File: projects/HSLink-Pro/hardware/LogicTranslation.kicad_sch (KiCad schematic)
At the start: 41 parts, among them U11 SN74LVC1T45DCK, U12 SN74LVC1T45DCK, U2 SN74LVC1T45DCK, U3 SN74LVC1T45DCK, U4 SN74LVC1T45DCK, U5 SN74LVC1T45DCK, U6 SN74LVC1T45DCK, U7 SN74LVC1T45DCK, U8 SN74LVC1T45DCK, U9 SN74LVC1T45DCK

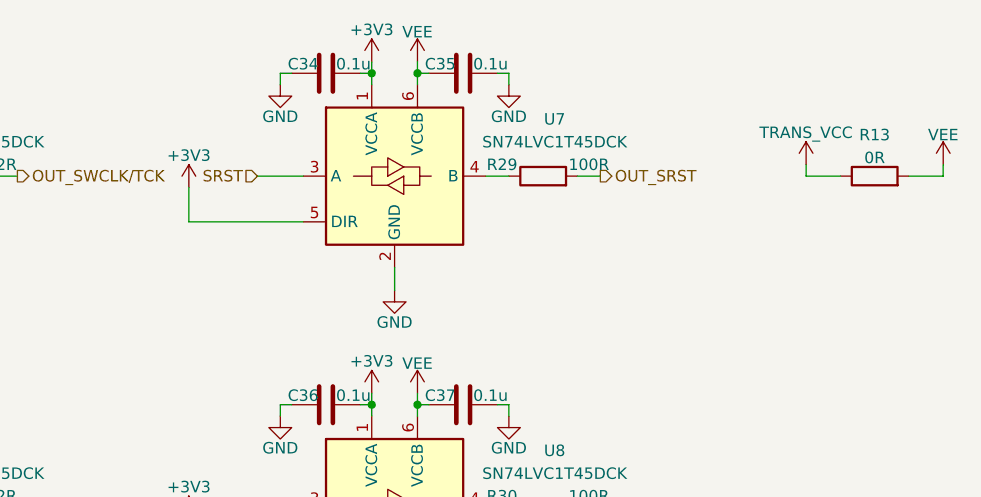
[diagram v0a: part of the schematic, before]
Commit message: update: 更新原理图
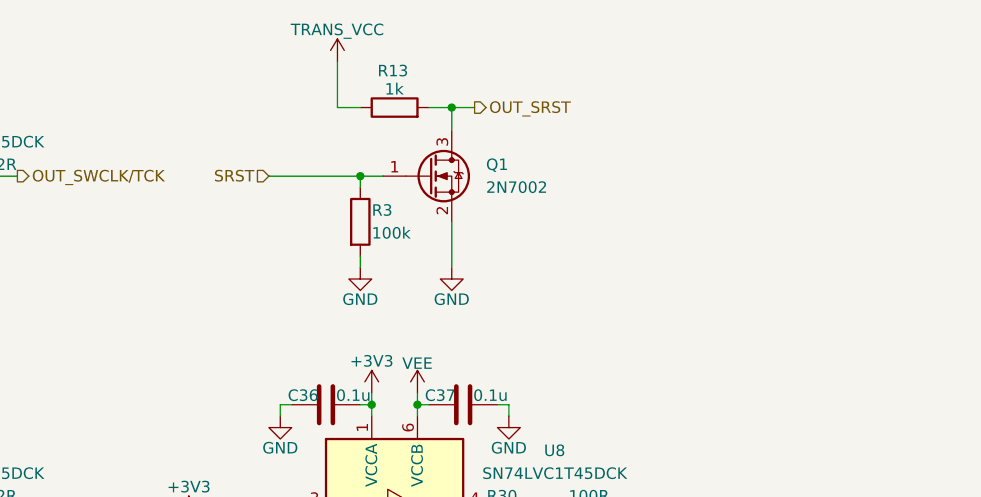
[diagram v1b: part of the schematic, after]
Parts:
- removed C34, C35: 0.1u, Capacitor_SMD:C_0402_1005Metric, symbol Device:C
- removed R29: 100R, Resistor_SMD:R_0402_1005Metric, symbol Device:R
- removed U7: SN74LVC1T45DCK, Package_TO_SOT_SMD:SOT-363_SC-70-6, symbol Logic_LevelTranslator:SN74LVC1T45DCK
- added Q1: 2N7002, Package_TO_SOT_SMD:SOT-323_SC-70, symbol Device:Q_NMOS_GSD
- added R3: 100k, Resistor_SMD:R_0402_1005Metric, symbol Device:R
- R13: value 0R -> 1k; footprint Resistor_SMD:R_0603_1608Metric -> Resistor_SMD:R_0402_1005Metric
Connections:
- net GND: now also Q1.2 (S), R3.2
- net OUT_SRST: now also R13.2, Q1.3 (D)
- net SRST: now also Q1.1 (G), R3.1
- net VEE: no longer R13.2
